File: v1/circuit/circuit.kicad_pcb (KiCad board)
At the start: 2 copper layers, 85 x 85 mm, 25 parts, among them J1 USB, J2 Conn_01x05_Male, J3 STEPPER, J5 LEDS, SW1 S_MODE, U1 TSR_1-2450, U3 4N35, U4 L293D

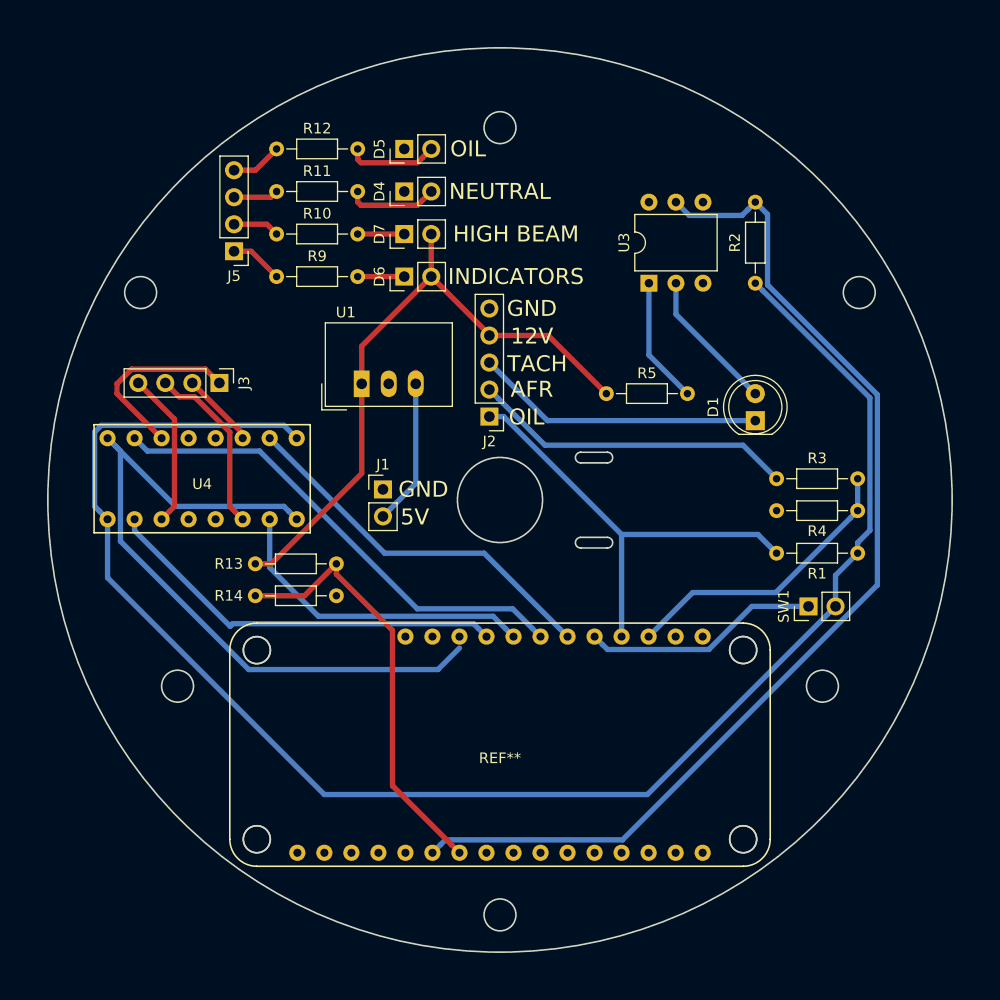
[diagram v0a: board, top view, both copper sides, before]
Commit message: Stuff
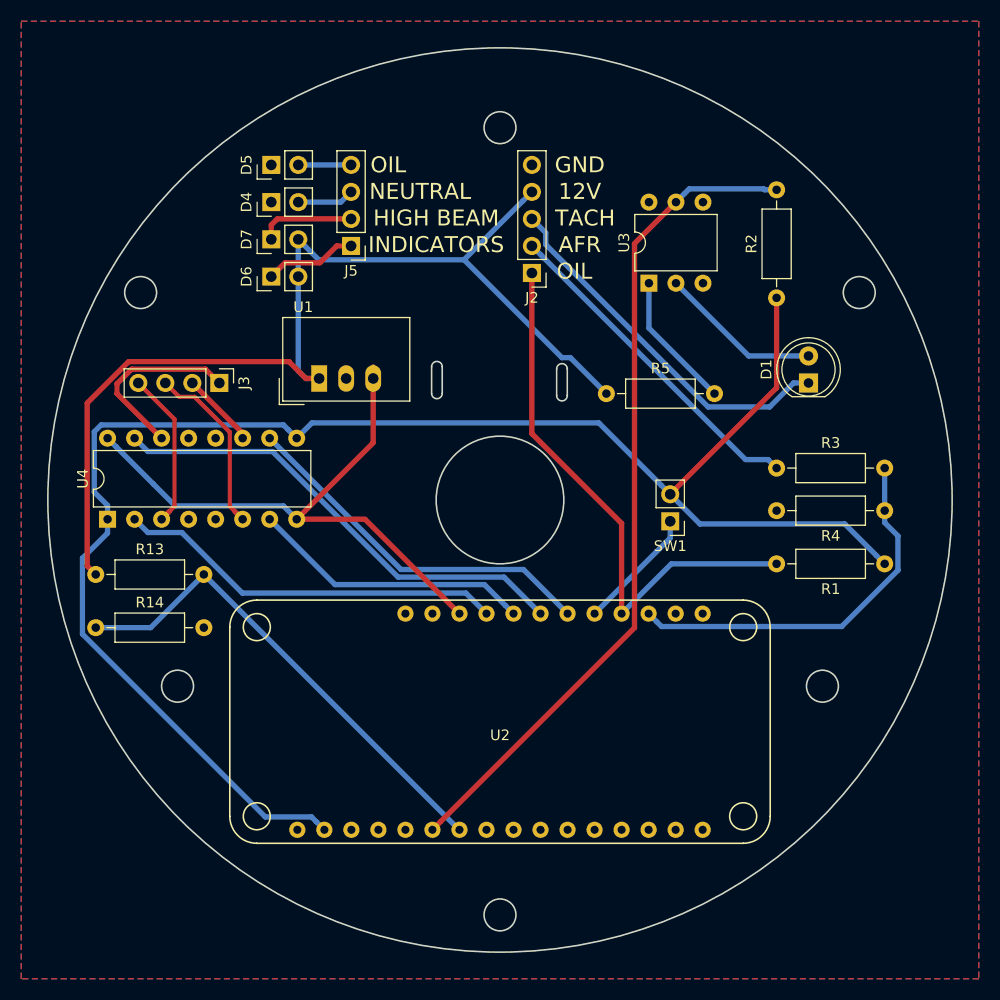
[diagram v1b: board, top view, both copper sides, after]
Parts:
- removed J1: USB, Connector_PinHeader_2.54mm:PinHeader_1x02_P2.54mm_Vertical
- removed R10, R11, R12, R9: 220, Resistor_THT:R_Axial_DIN0204_L3.6mm_D1.6mm_P7.62mm_Horizontal
- removed REF**: Feather, footprints:Feather
- added U2: Feather, footprints:Feather, F.Cu at (150.0, 120.8)
- R1, R13, R14, R3, R4: footprint Resistor_THT:R_Axial_DIN0204_L3.6mm_D1.6mm_P7.62mm_Horizontal -> Resistor_THT:R_Axial_DIN0207_L6.3mm_D2.5mm_P10.16mm_Horizontal
- R2: value 47k -> 20k; footprint Resistor_THT:R_Axial_DIN0204_L3.6mm_D1.6mm_P7.62mm_Horizontal -> Resistor_THT:R_Axial_DIN0207_L6.3mm_D2.5mm_P10.16mm_Horizontal
- R5: value 2k -> 1k; footprint Resistor_THT:R_Axial_DIN0204_L3.6mm_D1.6mm_P7.62mm_Horizontal -> Resistor_THT:R_Axial_DIN0207_L6.3mm_D2.5mm_P10.16mm_Horizontal
- U4: footprint Footprints:L293D -> Package_DIP:DIP-16_W7.62mm
- moved R14 15.3 mm to (112.0, 112.0)
- moved SW1 15.3 mm to (166.0, 102.0), turned to 180 degrees
- moved R13 15.0 mm to (112.0, 107.0)
- moved J2 14.1 mm to (153.0, 78.7)
- moved D5 12.6 mm to (128.5, 68.5)
- moved D4 12.5 mm to (128.5, 72.0)
- moved D7 12.5 mm to (128.5, 75.5)
- moved D6 12.5 mm to (128.5, 79.0)
- moved J5 11.0 mm to (136.0, 76.1)
- moved U4 9.67 mm to (113.1, 101.8), turned to 90 degrees
- moved D1 6.13 mm to (179.0, 89.0)
- moved U1 4.03 mm to (133.0, 88.6)
- moved R1 2.73 mm to (186.2, 106.0)
- moved R4 2.54 mm to (186.2, 101.0)
- moved R2 2.43 mm to (176.0, 81.0)
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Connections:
- J5 pad 1: Net-(J5-Pad1) -> Net-(D6-Pad1)
- J5 pad 2: Net-(J5-Pad2) -> Net-(D7-Pad1)
- J5 pad 3: Net-(J5-Pad3) -> Net-(D4-Pad2)
- J5 pad 4: Net-(J5-Pad4) -> Net-(D5-Pad2)
- SW1 pad 1: (no net) -> Net-(SW1-Pad1)
- U1 pad 3: Net-(J1-Pad2) -> +5V
- U4 pad 10: (no net) -> /STEP_4
- U4 pad 15: (no net) -> /STEP_3
- U4 pad 2: (no net) -> /STEP_1
- U4 pad 5: (no net) -> GND
- U4 pad 7: (no net) -> /STEP_2
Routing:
- net (no net): track 172.5 -> 0.00 mm
- net /STEP_3: track 0.00 -> 45.0 mm
- net +12V: track 59.8 -> 99.1 mm
- net /STEP_1: track 0.00 -> 36.8 mm
- net /STEP_4: track 0.00 -> 34.8 mm
- net /STEP_2: track 0.00 -> 26.6 mm
- net Net-(R2-Pad2): track 101.5 -> 78.5 mm
- net Net-(J1-Pad2): track 14.5 -> 0.00 mm
- net +5V: track 68.8 -> 56.9 mm
- net Net-(SW1-Pad1): track 0.00 -> 11.6 mm
- net Net-(J2-Pad1): track 41.9 -> 52.0 mm
- net Net-(R3-Pad2): track 27.6 -> 36.3 mm
- net Net-(D1-Pad1): track 27.3 -> 34.9 mm
- net Net-(R13-Pad2): track 40.8 -> 46.2 mm
- net Net-(J5-Pad1): track 4.99 -> 0.00 mm
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- added copper zone on B.Cu, net GND
- added copper zone on F.Cu, net GND
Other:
- outline, holes or cut-outs redrawn
- board text removed: "5V"
